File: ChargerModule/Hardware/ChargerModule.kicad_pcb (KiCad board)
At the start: 2 copper layers, 100 x 15 mm, 19 parts, among them J1 Connector, P1 1V8, T1 SI2333, T2 FDN337, T3 SI2333, U1 MCP73832, U2 NCP114 3V3, U3 MCP121

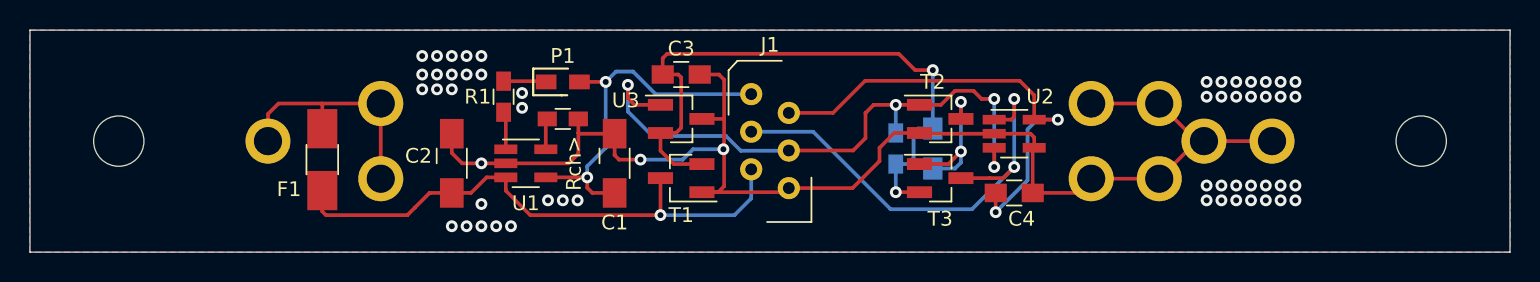
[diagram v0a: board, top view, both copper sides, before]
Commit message: Modifications
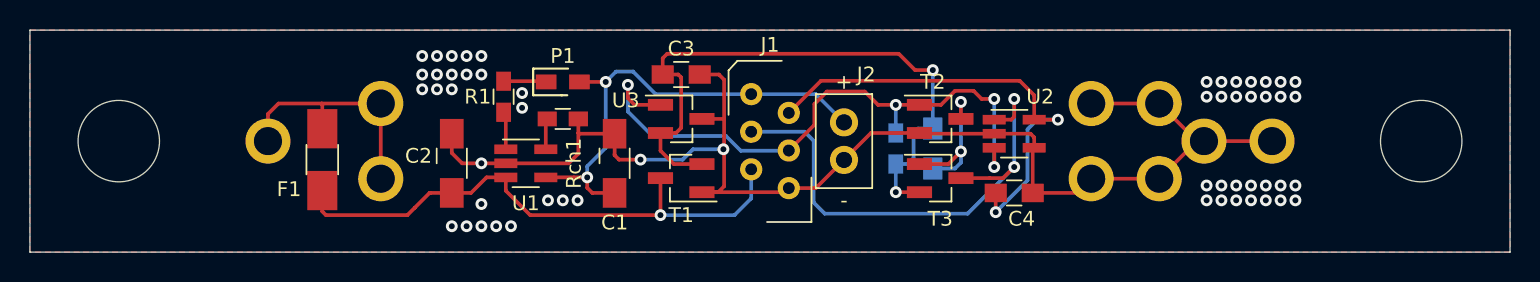
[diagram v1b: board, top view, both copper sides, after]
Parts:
- added J2: Power input, EsseivaN_Lib:WireConn_02, F.Cu at (155.0, 107.5)
- VIS_M3_88mm_space: footprint EsseivaN_Lib:VIS_M3_88mm -> EsseivaN_Lib:VIS_M5_88mm
- renumbered Rch> to Rch1
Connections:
- net GND_ALIM renamed GND
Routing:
- net /Vin: track 25.0 -> 32.0 mm
- net /VBAT: track 32.3 -> 35.0 mm
- net /~RST: track 41.6 -> 42.2 mm
- net GND: track 91.2 -> 90.6 mm
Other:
- board text added: "+"
- board text added: "-"
